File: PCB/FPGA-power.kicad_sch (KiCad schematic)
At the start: 13 parts, among them U1 XC7A50T-FGG484

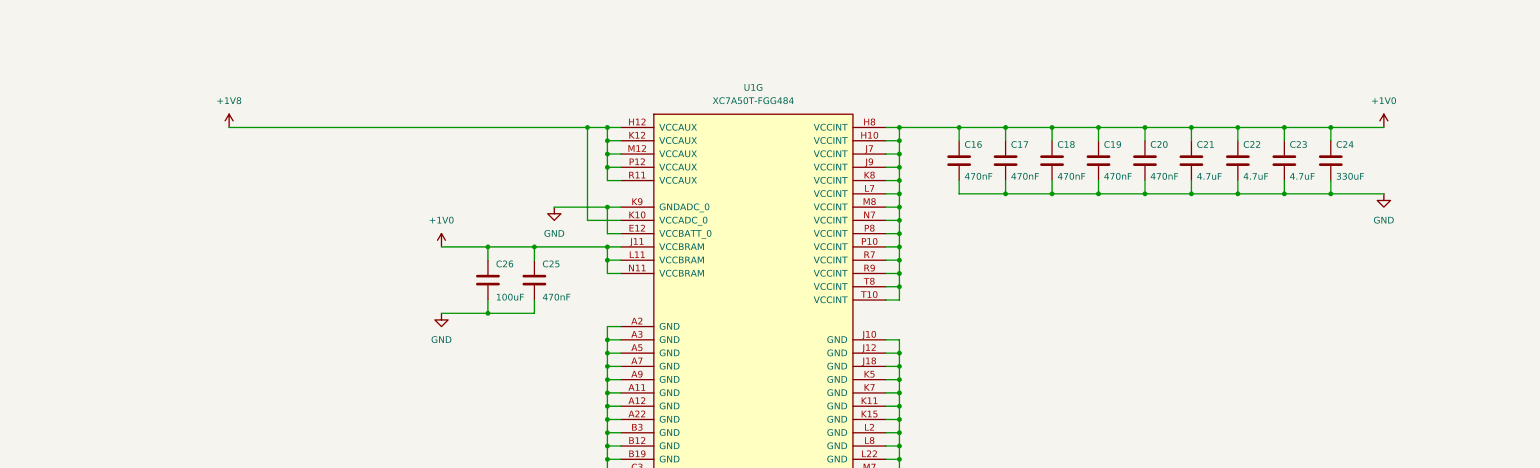
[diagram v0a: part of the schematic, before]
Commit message: VCCAUX decoupling
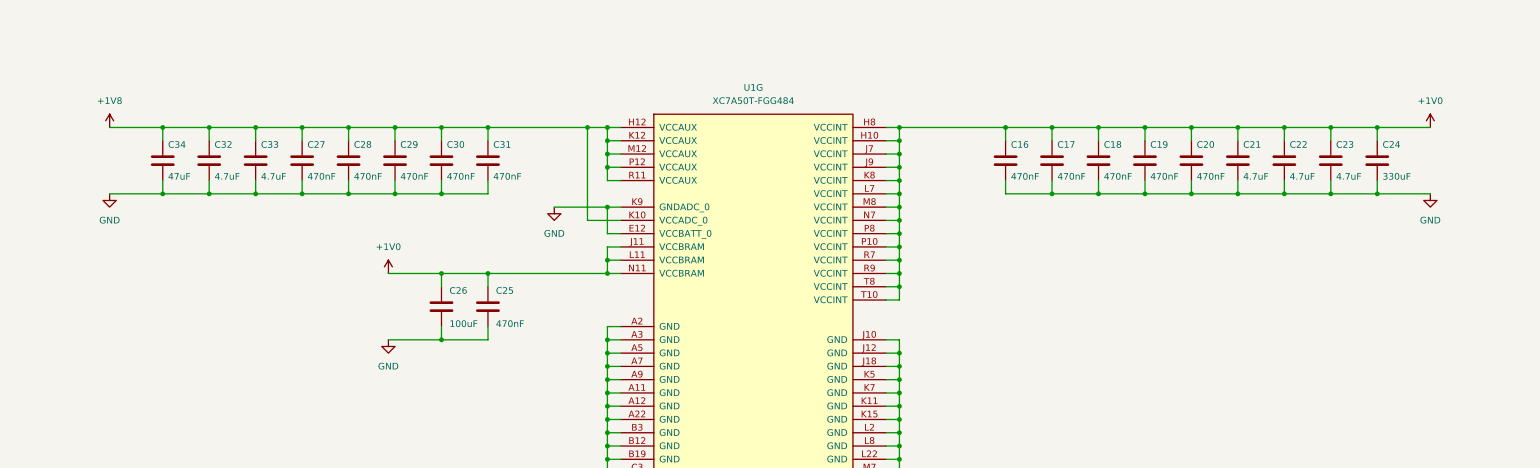
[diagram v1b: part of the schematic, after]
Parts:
- added C27, C28, C29, C30, C31: 470nF, symbol Device:C
- added C32, C33: 4.7uF, symbol Device:C
- added C34: 47uF, symbol Device:C
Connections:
- net +1V8: now also C27.1, C28.1, C29.1, C30.1, C31.1, C32.1, C33.1, C34.1
- net GND: now also C27.2, C28.2, C29.2, C30.2, C31.2, C32.2, C33.2, C34.2
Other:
- moved on the sheet: C16, C17, C18, C19, C20, C21, C22, C23, C24, C25, C26
